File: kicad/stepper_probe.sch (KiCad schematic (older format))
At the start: 55 parts, among them J1 Conn_01x04_Male, J2 Conn_01x04_Male, J3 BAT, J4 Serial Port, J5 SWD, J6 BAT, J7 Conn_01x01_Female, J8 Conn_01x01_Female, M1 Motor, SW1 SW_Push, U1 CC6920BSO-5A, U2 CC6920BSO-5A, U3 MDBT42Q-512KV2, U4 K7803MT-500R4, U5 M24C02-FMN, Y1 32.768Khz

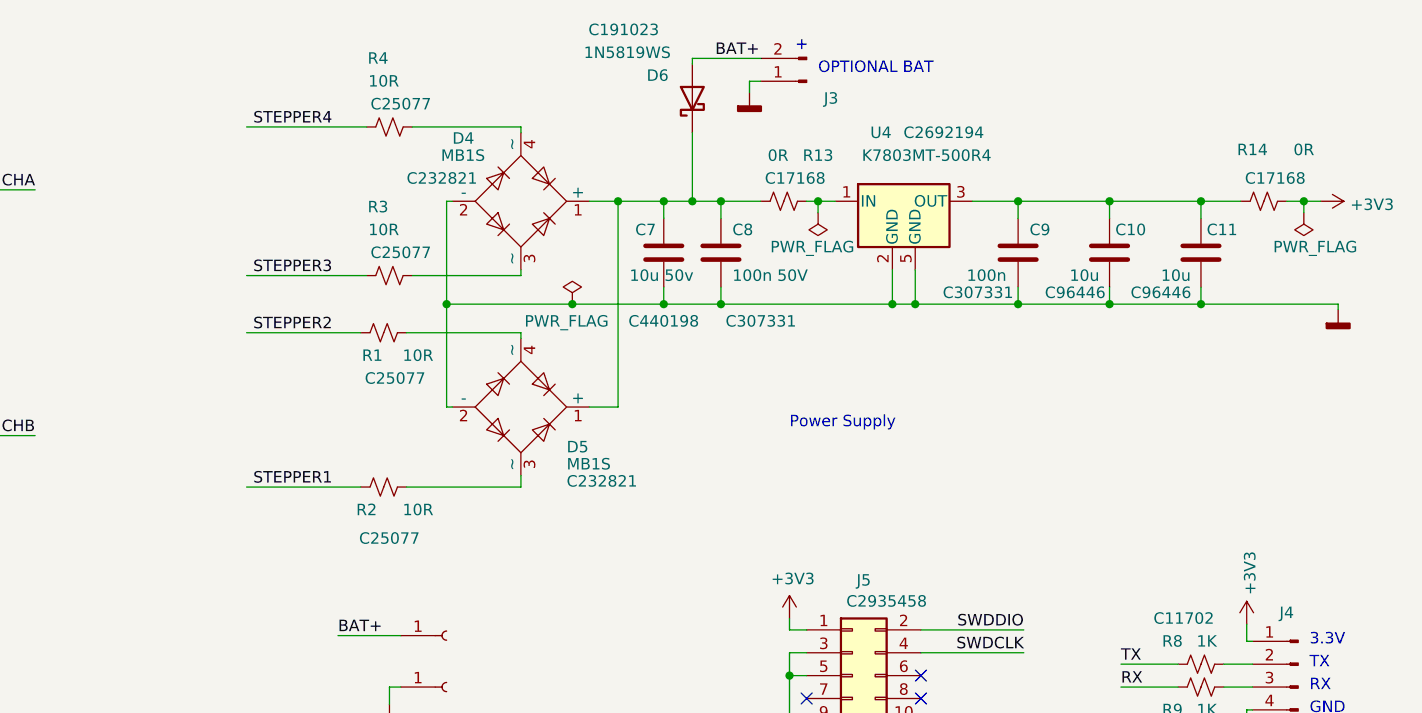
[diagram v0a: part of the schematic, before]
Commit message: Work in progress.
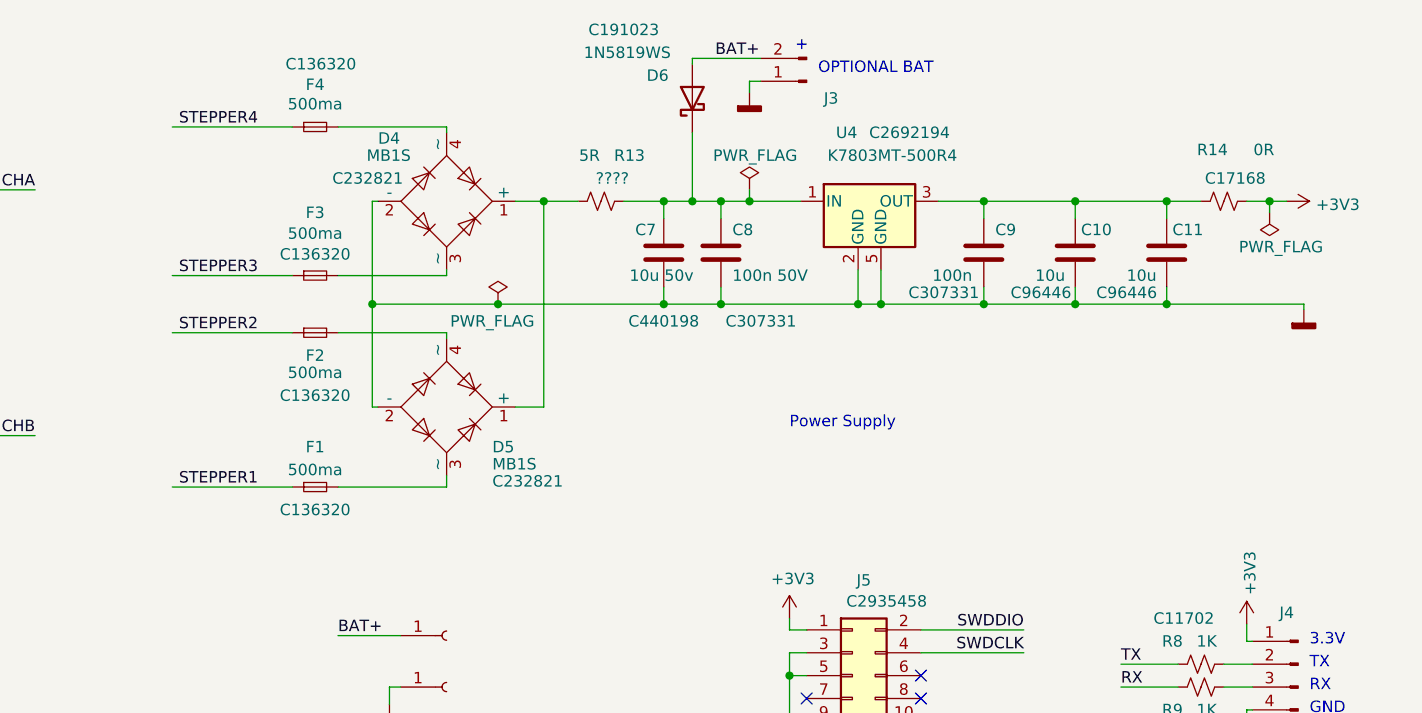
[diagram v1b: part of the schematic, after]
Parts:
- removed R1, R2, R3, R4: 10R, stepper_probe:R_0402_1005Metric_Pad0.72x0.64mm_HandSolder, symbol Device:R_Small_US
- added F1, F2, F3, F4: 500ma, stepper_probe:Fuse_0402, symbol Device:Fuse_Small
- R13: value 0R -> 5R; LCSC C17168 -> ????
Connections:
- net STEPPER1: now also F1.1
- net STEPPER2: now also F2.1
- net STEPPER3: now also F3.1
- net STEPPER4: now also F4.1
- net at D4.4 (~~): now also F4.2
- net at C7.1, C8.1, D6.1 (K): now also R13.1, U4.1 (IN); no longer D4.1 (+), D5.1 (+), R13.2
- net at D4.3 (~~): now also F3.2
- net at D5.3 (~~): now also F1.2
- net at D5.4 (~~): now also F2.2
- new net: D4.1 (+), D5.1 (+), R13.2
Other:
- moved on the sheet: C10, C11, C9, D4, D5, R13, R14, U4

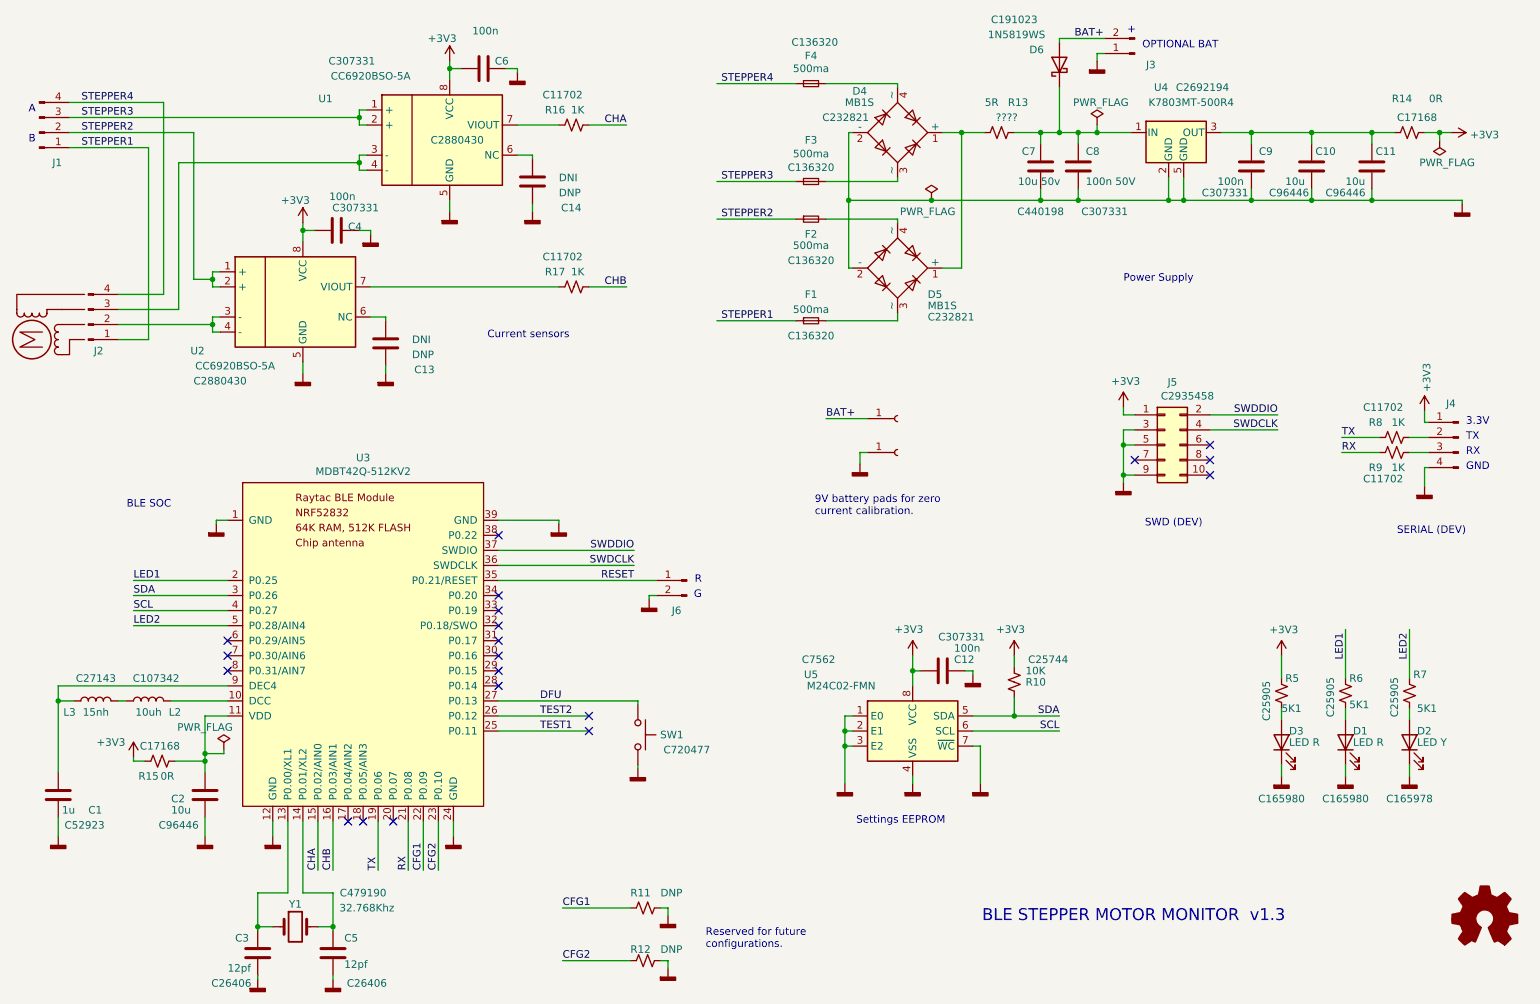
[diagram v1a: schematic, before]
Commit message: Minor clean ups.
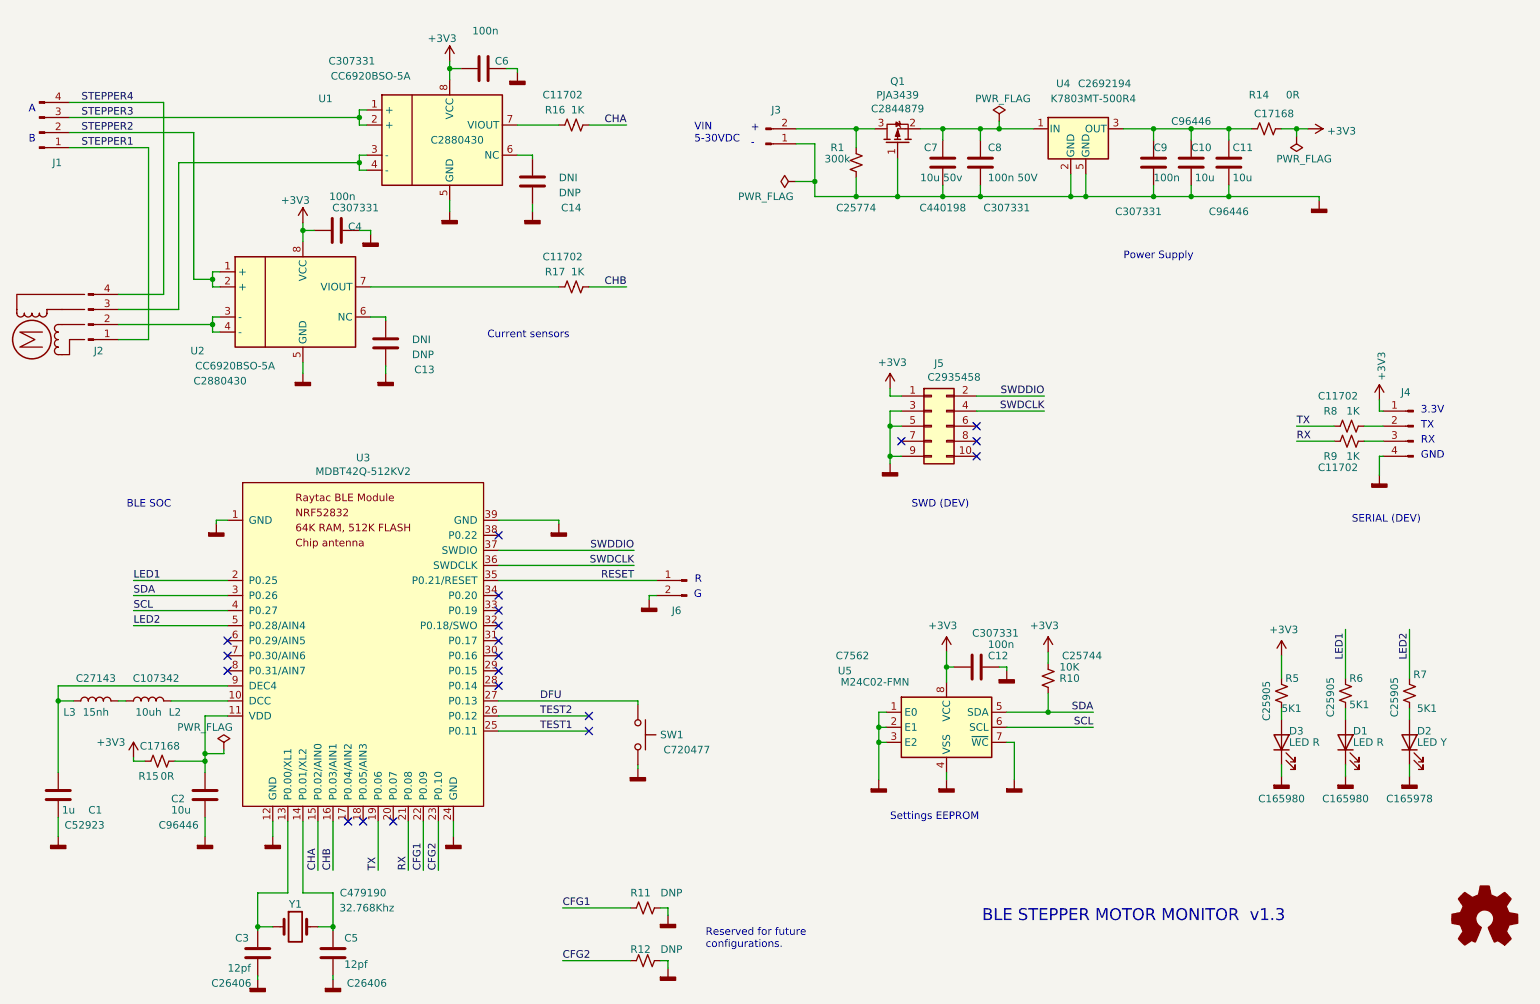
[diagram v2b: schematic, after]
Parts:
- removed D4, D5: MB1S, stepper_probe:DIODE_BRIDGE, symbol stepper_probe:DIODE_BRIDGE
- removed D6: 1N5819WS, stepper_probe:D_SOD-323_HandSoldering, symbol Device:D_Schottky
- removed F1, F2, F3, F4: 500ma, stepper_probe:Fuse_0402, symbol Device:Fuse_Small
- removed J7: Conn_01x01_Female, stepper_probe:BAT_PLUS_PAD, symbol Connector:Conn_01x01_Female
- removed J8: Conn_01x01_Female, stepper_probe:BAT_MINUS_PAD, symbol Connector:Conn_01x01_Female
- removed R13: 5R, stepper_probe:R_0402_1005Metric_Pad0.72x0.64mm_HandSolder, symbol Device:R_Small_US
- added Q1: PJA3439, Package_TO_SOT_SMD:SOT-23, symbol stepper_probe:P_MOSFET
- added R1: 300k, stepper_probe:R_0402_1005Metric_Pad0.72x0.64mm_HandSolder, symbol Device:R_Small_US
- J3: footprint stepper_probe:PinHeader_1x02_P2.54mm_Vertical -> stepper_probe:connector_2pins_horizontal; LCSC (none) -> C30436
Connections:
- net GND: now also Q1.1 (G), R1.1
- net at C7.1, C8.1, U4.1 (IN): now also Q1.2 (S)
- net BAT+: no longer names the net of J3.2 (Pin_2)
- net BAT+: now also Q1.3 (D), R1.2
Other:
- note added: "-"
- note added: "VIN\n5-30VDC"
- note removed: "9V battery pads for zero \ncurrent calibration."
- note removed: "OPTIONAL BAT"
- moved on the sheet: C10, C11, C12, C7, C8, C9, J3, J4, J5, R10, R14, R8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
